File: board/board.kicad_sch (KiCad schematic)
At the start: 1 part

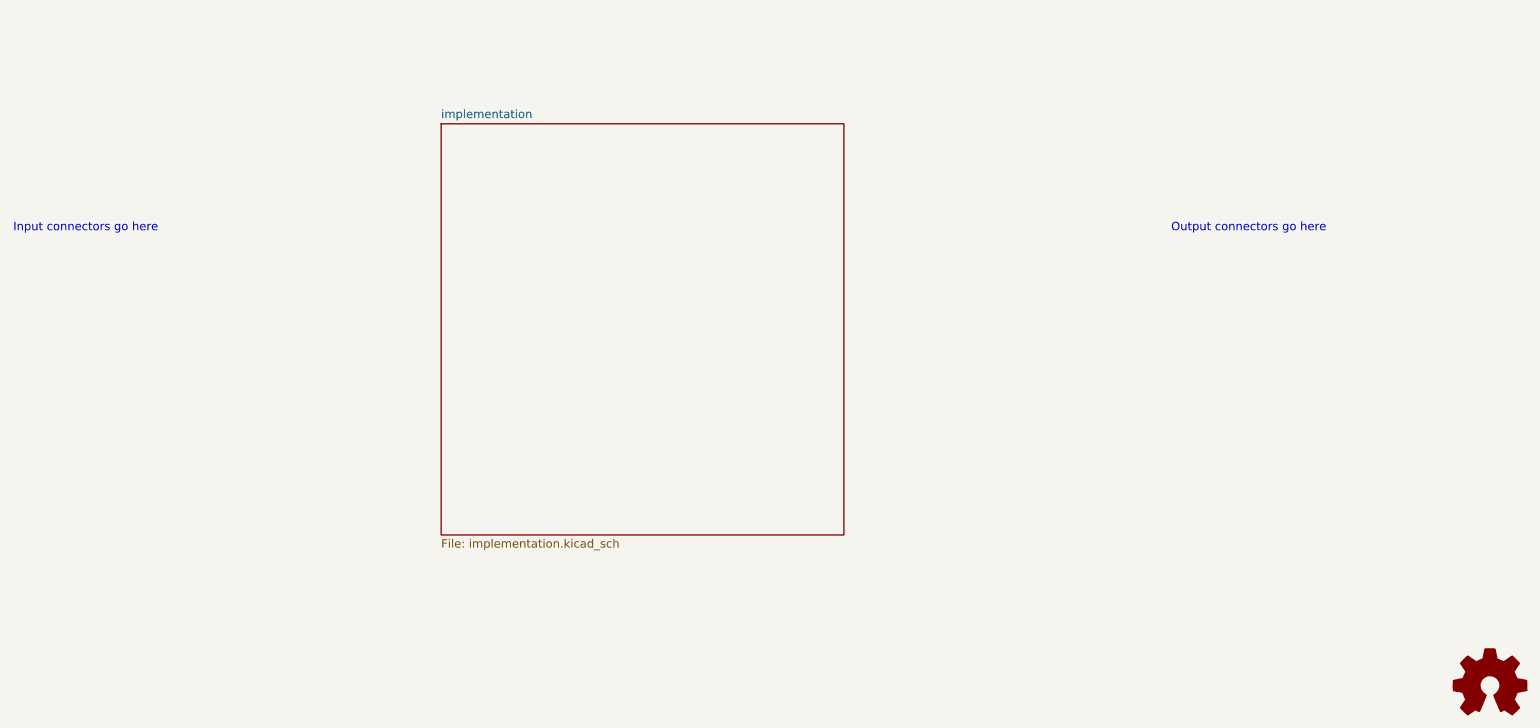
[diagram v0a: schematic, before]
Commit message: initial
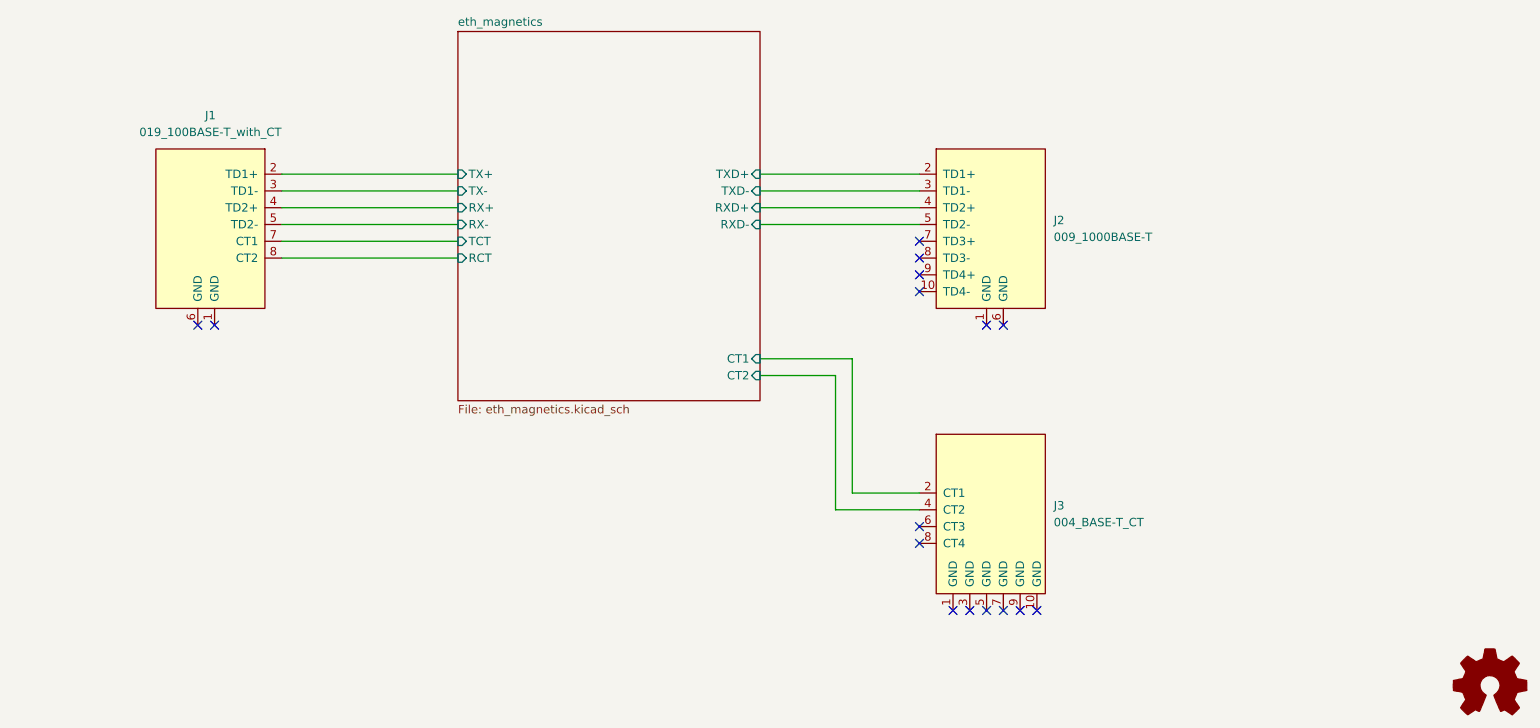
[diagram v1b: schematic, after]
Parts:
- added J1: 019_100BASE-T_with_CT, on_edge:on_edge_2x05_device, symbol put_on_edge:019_100BASE-T_with_CT
- added J2: 009_1000BASE-T, on_edge:on_edge_2x05_host, symbol put_on_edge:009_1000BASE-T
- added J3: 004_BASE-T_CT, on_edge:on_edge_2x05_host, symbol put_on_edge:004_BASE-T_CT
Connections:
- new net eth_magnetics/CT1: J3.2 (CT1)
- new net eth_magnetics/CT2: J3.4 (CT2)
- new net eth_magnetics/RCT: J1.8 (CT2)
- new net eth_magnetics/RX+: J1.4 (TD2+)
- new net eth_magnetics/RX-: J1.5 (TD2-)
- new net eth_magnetics/RXD+: J2.4 (TD2+)
- new net eth_magnetics/RXD-: J2.5 (TD2-)
- new net eth_magnetics/TCT: J1.7 (CT1)
- new net eth_magnetics/TX+: J1.2 (TD1+)
- new net eth_magnetics/TX-: J1.3 (TD1-)
- new net eth_magnetics/TXD+: J2.2 (TD1+)
- new net eth_magnetics/TXD-: J2.3 (TD1-)
- no-connect marks 0 -> 16
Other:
- removed sheet implementation
- added sheet eth_magnetics (eth_magnetics.kicad_sch)
- note removed: "Input connectors go here"
- note removed: "Output connectors go here"
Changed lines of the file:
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@@
 (kicad_sch (version 20211123) (generator eeschema)
   (paper "A4")
-  (text "Output connectors go here" (at 224.79 88.9 0)
-    (effects (font (size 1.27 1.27)) (justify left bottom))
-  )
-  (text "Input connectors go here" (at 49.53 88.9 0)
-    (effects (font (size 1.27 1.27)) (justify left bottom))
+  (no_connect (at 80.01 102.87))
+  (no_connect (at 77.47 102.87))
+  (no_connect (at 186.69 90.17))
+  (no_connect (at 186.69 95.25))
+  (no_connect (at 186.69 92.71))
+  (no_connect (at 186.69 97.79))
+  (no_connect (at 204.47 146.05))
+  (no_connect (at 194.31 146.05))
+  (no_connect (at 196.85 146.05))
+  (no_connect (at 199.39 146.05))
+  (no_connect (at 201.93 146.05))
+  (no_connect (at 199.39 102.87))
+  (no_connect (at 196.85 102.87))
+  (no_connect (at 191.77 146.05))
+  (no_connect (at 186.69 135.89))
+  (no_connect (at 186.69 133.35))
+  (wire (pts (xy 173.99 130.81) (xy 186.69 130.81))
+    (stroke (width 0) (type default) (color 0 0 0 0))
+  )
+  (wire (pts (xy 90.17 82.55) (xy 116.84 82.55))
+    (stroke (width 0) (type default) (color 0 0 0 0))
+  )
+  (wire (pts (xy 162.56 85.09) (xy 186.69 85.09))
+    (stroke (width 0) (type default) (color 0 0 0 0))
+  )
+  (wire (pts (xy 162.56 82.55) (xy 186.69 82.55))
+    (stroke (width 0) (type default) (color 0 0 0 0))
+  )
+  (wire (pts (xy 162.56 107.95) (xy 176.53 107.95))
+    (stroke (width 0) (type default) (color 0 0 0 0))
+  )
+  (wire (pts (xy 176.53 128.27) (xy 186.69 128.27))
+    (stroke (width 0) (type default) (color 0 0 0 0))
+  )
+  (wire (pts (xy 162.56 87.63) (xy 186.69 87.63))
+    (stroke (width 0) (type default) (color 0 0 0 0))
+  )
+  (wire (pts (xy 90.17 92.71) (xy 116.84 92.71))
+    (stroke (width 0) (type default) (color 0 0 0 0))
+  )
+  (wire (pts (xy 90.17 90.17) (xy 116.84 90.17))
+    (stroke (width 0) (type default) (color 0 0 0 0))
+  )
+  (wire (pts (xy 176.53 107.95) (xy 176.53 128.27))
+    (stroke (width 0) (type default) (color 0 0 0 0))
+  )
+  (wire (pts (xy 90.17 80.01) (xy 116.84 80.01))
+    (stroke (width 0) (type default) (color 0 0 0 0))
+  )
+  (wire (pts (xy 162.56 110.49) (xy 173.99 110.49))
+    (stroke (width 0) (type default) (color 0 0 0 0))
+  )
+  (wire (pts (xy 173.99 110.49) (xy 173.99 130.81))
+    (stroke (width 0) (type default) (color 0 0 0 0))
+  )
+  (wire (pts (xy 90.17 87.63) (xy 116.84 87.63))
+    (stroke (width 0) (type default) (color 0 0 0 0))
+  )
+  (wire (pts (xy 90.17 85.09) (xy 116.84 85.09))
+    (stroke (width 0) (type default) (color 0 0 0 0))
+  )
+  (wire (pts (xy 162.56 80.01) (xy 186.69 80.01))
+    (stroke (width 0) (type default) (color 0 0 0 0))
   )
   (symbol (lib_id "Graphic:Logo_Open_Hardware_Small") (at 273.05 157.48 0) (unit 1)
@@
     )
   )
-  (sheet (at 114.3 72.39) (size 60.96 62.23) (fields_autoplaced)
+  (symbol (lib_id "put_on_edge:004_BASE-T_CT") (at 198.12 132.08 0) (unit 1)
+    (in_bom yes) (on_board yes) (fields_autoplaced)
+    (property "Reference" "J3" (id 0) (at 207.01 130.1749 0)
+      (effects (font (size 1.27 1.27)) (justify left))
+    )
+    (property "Value" "004_BASE-T_CT" (id 1) (at 207.01 132.7149 0)
+      (effects (font (size 1.27 1.27)) (justify left))
+    )
+    (property "Footprint" "on_edge:on_edge_2x05_host" (id 2) (at 205.74 115.57 0)
+      (effects (font (size 1.27 1.27)) hide)
+    )
+    (property "Datasheet" "" (id 3) (at 205.74 115.57 0)
+      (effects (font (size 1.27 1.27)) hide)
+    )
+    (pin "1")
+    (pin "10")
+    (pin "2")
+    (pin "3")
+    (pin "4")
+    (pin "5")
+    (pin "6")
+    (pin "7")
+    (pin "8")
+    (pin "9")
+  )
+  (symbol (lib_id "put_on_edge:019_100BASE-T_with_CT") (at 78.74 88.9 0) (mirror y) (unit 1)
+    (in_bom yes) (on_board yes) (fields_autoplaced)
+    (property "Reference" "J1" (id 0) (at 79.375 71.12 0))
+    (property "Value" "019_100BASE-T_with_CT" (id 1) (at 79.375 73.66 0))
+    (property "Footprint" "on_edge:on_edge_2x05_device" (id 2) (at 71.12 72.39 0)
+      (effects (font (size 1.27 1.27)) hide)
+    )
+    (property "Datasheet" "" (id 3) (at 71.12 72.39 0)
+      (effects (font (size 1.27 1.27)) hide)
+    )
+    (pin "1")
+    (pin "2")
+    (pin "3")
+    (pin "4")
+    (pin "5")
+    (pin "6")
+    (pin "7")
+    (pin "8")
+  )
+  (symbol (lib_id "put_on_edge:009_1000BASE-T") (at 198.12 88.9 0) (unit 1)
+    (in_bom yes) (on_board yes) (fields_autoplaced)
+    (property "Reference" "J2" (id 0) (at 207.01 86.9949 0)
+      (effects (font (size 1.27 1.27)) (justify left))
+    )
+    (property "Value" "009_1000BASE-T" (id 1) (at 207.01 89.5349 0)
+      (effects (font (size 1.27 1.27)) (justify left))
+    )
+    (property "Footprint" "on_edge:on_edge_2x05_host" (id 2) (at 205.74 72.39 0)
+      (effects (font (size 1.27 1.27)) hide)
+    )
+    (property "Datasheet" "" (id 3) (at 205.74 72.39 0)
+      (effects (font (size 1.27 1.27)) hide)
+    )
+    (pin "1")
+    (pin "10")
+    (pin "2")
+    (pin "3")
+    (pin "4")
+    (pin "5")
+    (pin "6")
+    (pin "7")
+    (pin "8")
+    (pin "9")
+  )
+  (sheet (at 116.84 58.42) (size 45.72 55.88) (fields_autoplaced)
     (stroke (width 0.1524) (type solid) (color 0 0 0 0))
     (fill (color 0 0 0 0.0000))
-    (property "Sheet name" "implementation" (id 0) (at 114.3 71.6784 0)
+    (property "Sheet name" "eth_magnetics" (id 0) (at 116.84 57.7084 0)
       (effects (font (size 1.27 1.27)) (justify left bottom))
     )
-    (property "Sheet file" "implementation.kicad_sch" (id 1) (at 114.3 135.2046 0)
+    (property "Sheet file" "eth_magnetics.kicad_sch" (id 1) (at 116.84 114.8846 0)
       (effects (font (size 1.27 1.27)) (justify left top))
+    )
+    (pin "CT1" input (at 162.56 107.95 0)
+      (effects (font (size 1.27 1.27)) (justify right))
+    )
+    (pin "TXD-" input (at 162.56 82.55 0)
+      (effects (font (size 1.27 1.27)) (justify right))
+    )
+    (pin "TXD+" input (at 162.56 80.01 0)
+      (effects (font (size 1.27 1.27)) (justify right))
+    )
+    (pin "RXD+" input (at 162.56 85.09 0)
+      (effects (font (size 1.27 1.27)) (justify right))
+    )
+    (pin "CT2" input (at 162.56 110.49 0)
+      (effects (font (size 1.27 1.27)) (justify right))
+    )
+    (pin "RXD-" input (at 162.56 87.63 0)
+      (effects (font (size 1.27 1.27)) (justify right))
+    )
+    (pin "RCT" input (at 116.84 92.71 180)
+      (effects (font (size 1.27 1.27)) (justify left))
+    )
+    (pin "TX-" input (at 116.84 82.55 180)
+      (effects (font (size 1.27 1.27)) (justify left))
+    )
+    (pin "RX+" input (at 116.84 85.09 180)
+      (effects (font (size 1.27 1.27)) (justify left))
+    )
+    (pin "RX-" input (at 116.84 87.63 180)
+      (effects (font (size 1.27 1.27)) (justify left))
+    )
+    (pin "TX+" input (at 116.84 80.01 180)
+      (effects (font (size 1.27 1.27)) (justify left))
+    )
+    (pin "TCT" input (at 116.84 90.17 180)
+      (effects (font (size 1.27 1.27)) (justify left))
     )
   )
   (sheet_instances
     (path "/" (page "1"))
-    (path "/767ce4c6-0e55-4543-92f0-34cb8237a544" (page "2"))
+    (path "/3c188f4a-96b0-46fe-81a4-4bc44d10569e" (page "2"))
   )
   (symbol_instances
+    (path "/df2e3995-6ff2-4214-8b56-2b5f6b2926fa"
+      (reference "J1") (unit 1) (value "019_100BASE-T_with_CT") (footprint "on_edge:on_edge_2x05_device")
+    )
+    (path "/e3915cad-b4f2-4bb4-9c5d-5d2f91f3e569"
+      (reference "J2") (unit 1) (value "009_1000BASE-T") (footprint "on_edge:on_edge_2x05_host")
+    )
+    (path "/b78e9d36-43ff-4cc7-ab50-e83113c69f50"
+      (reference "J3") (unit 1) (value "004_BASE-T_CT") (footprint "on_edge:on_edge_2x05_host")
+    )
     (path "/b72b6f4a-7489-40f2-bb90-d75ae01aa368"
       (reference "LOGO1") (unit 1) (value "Logo_Open_Hardware_Small") (footprint "Symbol:OSHW-Symbol_6.7x6mm_SilkScreen")
     )
-  )
+    (path "/3c188f4a-96b0-46fe-81a4-4bc44d10569e/945b33c5-49a8-444d-b505-546d6d2125e5"
+      (reference "TR1") (unit 1) (value "749013011A") (footprint "b099:749013011A")
+    )
+  )
